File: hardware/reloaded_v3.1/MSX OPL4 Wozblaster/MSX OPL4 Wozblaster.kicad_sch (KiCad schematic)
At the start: 34 parts, among them IC1 GAL16V8D, IC2 KM684000ALG, IC3 KM684000ALG, IC4 NJM4558, IC5 YMF278B-F, IC6 AM29F016B-120EC, Q1 33.8688, SW1 SW_Push, U1 KCX_BT_EMITTER, U2 UDA1334MOD

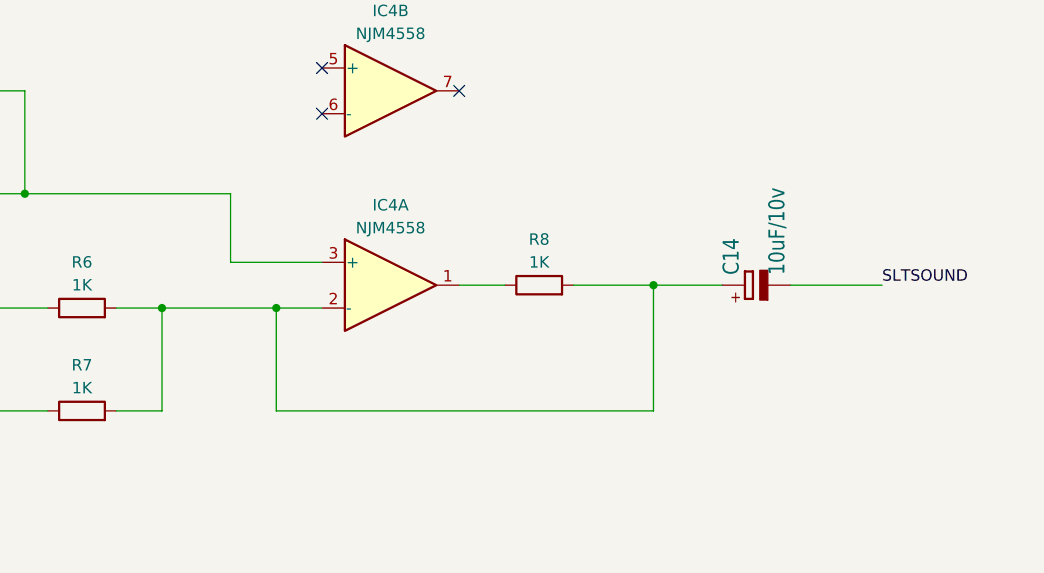
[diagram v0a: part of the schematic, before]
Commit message: v3.2
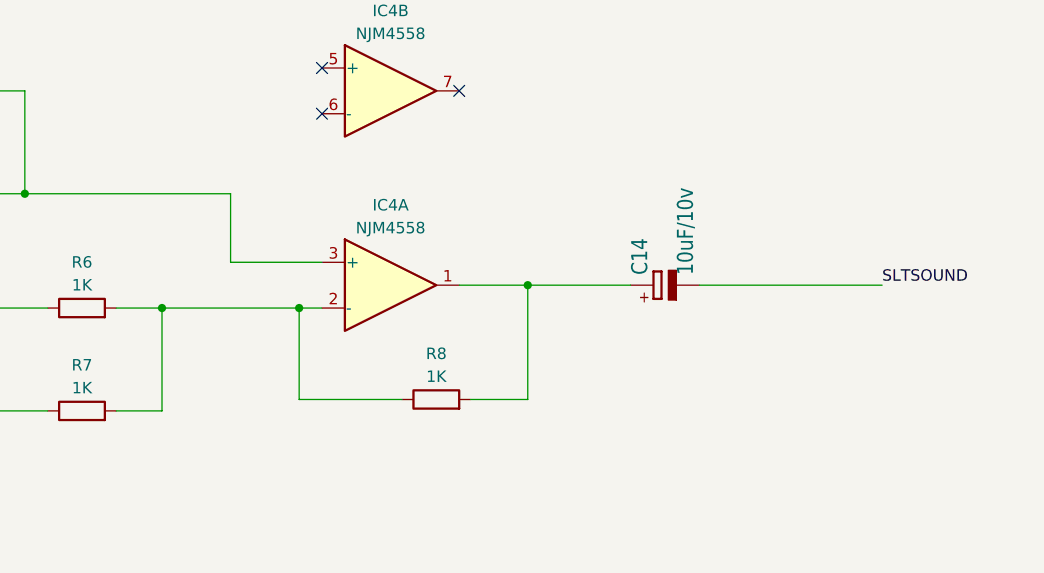
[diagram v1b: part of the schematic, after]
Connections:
- net at IC4.1: now also C14.1 (+), R8.2; no longer R8.1
- net at IC4.2 (-), R6.2, R7.2: now also R8.1; no longer C14.1 (+), R8.2
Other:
- moved on the sheet: C14
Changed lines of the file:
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@@
     (comment 4 "Wozblaster Reloaded v3")
   )
+  (junction (at 452.12 252.73) (diameter 0) (color 0 0 0 0)
+  )
   (junction (at 157.48 288.29) (diameter 0) (color 0 0 0 0)
   )
@@
   (junction (at 234.95 139.7) (diameter 0) (color 0 0 0 0)
   )
-  (junction (at 449.58 252.73) (diameter 0) (color 0 0 0 0)
-  )
   (junction (at 200.66 149.86) (diameter 0) (color 0 0 0 0)
   )
+  (junction (at 477.52 250.19) (diameter 0) (color 0 0 0 0)
+  )
   (junction (at 224.79 118.11) (diameter 0) (color 0 0 0 0)
   )
@@
   (junction (at 234.95 152.4) (diameter 0) (color 0 0 0 0)
   )
-  (junction (at 491.49 250.19) (diameter 0) (color 0 0 0 0)
-  )
   (junction (at 214.63 118.11) (diameter 0) (color 0 0 0 0)
   )
@@
     (stroke (width 0) (type default))
   )
-  (wire (pts (xy 436.88 252.73) (xy 449.58 252.73))
+  (wire (pts (xy 436.88 252.73) (xy 452.12 252.73))
     (stroke (width 0) (type default))
   )
@@
     (stroke (width 0) (type default))
   )
+  (wire (pts (xy 471.17 262.89) (xy 477.52 262.89))
+    (stroke (width 0) (type default))
+  )
   (wire (pts (xy 421.64 228.6) (xy 421.64 240.03))
     (stroke (width 0) (type default))
@@
     (stroke (width 0) (type default))
   )
-  (wire (pts (xy 491.49 250.19) (xy 499.11 250.19))
-    (stroke (width 0) (type default))
-  )
   (wire (pts (xy 396.24 228.6) (xy 405.13 228.6))
     (stroke (width 0) (type default))
@@
     (stroke (width 0) (type default))
   )
+  (wire (pts (xy 452.12 262.89) (xy 463.55 262.89))
+    (stroke (width 0) (type default))
+  )
   (wire (pts (xy 496.57 76.2) (xy 502.92 76.2))
     (stroke (width 0) (type default))
@@
     (stroke (width 0) (type default))
   )
+  (wire (pts (xy 477.52 250.19) (xy 488.95 250.19))
+    (stroke (width 0) (type default))
+  )
   (wire (pts (xy 273.05 147.32) (xy 278.13 147.32))
     (stroke (width 0) (type default))
@@
     (stroke (width 0) (type default))
   )
-  (wire (pts (xy 469.9 250.19) (xy 474.98 250.19))
+  (wire (pts (xy 469.9 250.19) (xy 477.52 250.19))
     (stroke (width 0) (type default))
   )
@@
     (stroke (width 0) (type default))
   )
-  (wire (pts (xy 482.6 250.19) (xy 491.49 250.19))
-    (stroke (width 0) (type default))
-  )
   (wire (pts (xy 273.05 109.22) (xy 278.13 109.22))
     (stroke (width 0) (type default))
@@
     (stroke (width 0) (type default))
   )
+  (wire (pts (xy 477.52 262.89) (xy 477.52 250.19))
+    (stroke (width 0) (type default))
+  )
   (wire (pts (xy 132.08 270.51) (xy 127 270.51))
     (stroke (width 0) (type default))
@@
     (stroke (width 0) (type default))
   )
-  (wire (pts (xy 506.73 250.19) (xy 516.89 250.19))
-    (stroke (width 0) (type default))
-  )
   (wire (pts (xy 381 273.05) (xy 387.35 273.05))
     (stroke (width 0) (type default))
@@
     (stroke (width 0) (type default))
   )
-  (wire (pts (xy 491.49 250.19) (xy 491.49 264.16))
-    (stroke (width 0) (type default))
-  )
   (wire (pts (xy 217.17 54.61) (xy 229.87 54.61))
     (stroke (width 0) (type default))
@@
     (stroke (width 0) (type default))
   )
+  (wire (pts (xy 452.12 252.73) (xy 454.66 252.73))
+    (stroke (width 0) (type default))
+  )
   (wire (pts (xy 314.96 118.11) (xy 321.31 118.11))
     (stroke (width 0) (type default))
@@
     (stroke (width 0) (type default))
   )
-  (wire (pts (xy 449.58 264.16) (xy 449.58 252.73))
+  (wire (pts (xy 452.12 252.73) (xy 452.12 262.89))
     (stroke (width 0) (type default))
   )
@@
     (stroke (width 0) (type default))
   )
-  (wire (pts (xy 449.58 252.73) (xy 454.66 252.73))
-    (stroke (width 0) (type default))
-  )
   (wire (pts (xy 381 270.51) (xy 383.54 270.51))
     (stroke (width 0) (type default))
@@
     (stroke (width 0) (type default))
   )
-  (wire (pts (xy 491.49 264.16) (xy 449.58 264.16))
-    (stroke (width 0) (type default))
-  )
   (wire (pts (xy 273.05 269.24) (xy 285.75 269.24))
     (stroke (width 0) (type default))
@@
     (stroke (width 0) (type default))
   )
+  (wire (pts (xy 496.57 250.19) (xy 516.89 250.19))
+    (stroke (width 0) (type default))
+  )
   (wire (pts (xy 496.57 81.28) (xy 502.92 81.28))
     (stroke (width 0) (type default))
@@
     )
   )
-  (symbol (lib_id "Device:R") (at 478.79 250.19 90) (unit 1)
-    (in_bom yes) (on_board yes) (dnp no) (fields_autoplaced)
-    (property "Reference" "R8" (at 478.79 245.11 90)
-      (effects (font (size 1.27 1.27)))
-    )
-    (property "Value" "1K" (at 478.79 247.65 90)
-      (effects (font (size 1.27 1.27)))
-    )
-    (property "Footprint" "Resistor_SMD:R_0603_1608Metric" (at 478.79 251.968 90)
-      (effects (font (size 1.27 1.27)) hide)
-    )
-    (property "Datasheet" "~" (at 478.79 250.19 0)
-      (effects (font (size 1.27 1.27)) hide)
-    )
-    (pin "1")
-    (pin "2")
-    (instances
-      (project "MSX OPL4 Wozblaster"
-        (path "/319085e4-dbf0-404d-8e32-9614d4e1a0c6"
-          (reference "R8") (unit 1)
-        )
-      )
-    )
-  )
   (symbol (lib_id "power:GND") (at 90.17 293.37 0) (unit 1)
     (in_bom yes) (on_board yes) (dnp no) (fields_autoplaced)
@@
     )
   )
+  (symbol (lib_id "Device:R") (at 467.36 262.89 90) (unit 1)
+    (in_bom yes) (on_board yes) (dnp no) (fields_autoplaced)
+    (property "Reference" "R8" (at 467.36 257.81 90)
+      (effects (font (size 1.27 1.27)))
+    )
+    (property "Value" "1K" (at 467.36 260.35 90)
+      (effects (font (size 1.27 1.27)))
+    )
+    (property "Footprint" "Resistor_SMD:R_0603_1608Metric" (at 467.36 264.668 90)
+      (effects (font (size 1.27 1.27)) hide)
+    )
+    (property "Datasheet" "~" (at 467.36 262.89 0)
+      (effects (font (size 1.27 1.27)) hide)
+    )
+    (pin "1")
+    (pin "2")
+    (instances
+      (project "MSX OPL4 Wozblaster"
+        (path "/319085e4-dbf0-404d-8e32-9614d4e1a0c6"
+          (reference "R8") (unit 1)
+        )
+      )
+    )
+  )
   (symbol (lib_id "CRISAG:C-EU") (at 208.28 118.11 270) (unit 1)
     (in_bom yes) (on_board yes) (dnp no)
@@
     )
   )
-  (symbol (lib_id "CRISAG:CPOLSMCB") (at 501.65 250.19 90) (unit 1)
+  (symbol (lib_id "CRISAG:CPOLSMCB") (at 491.49 250.19 90) (unit 1)
     (in_bom yes) (on_board yes) (dnp no)
-    (property "Reference" "C14" (at 501.1674 249.047 0)
+    (property "Reference" "C14" (at 491.0074 249.047 0)
       (effects (font (size 1.778 1.5113)) (justify left bottom))
     )
-    (property "Value" "10uF/10v" (at 506.2474 249.047 0)
+    (property "Value" "10uF/10v" (at 496.0874 249.047 0)
       (effects (font (size 1.778 1.5113)) (justify left bottom))
     )
-    (property "Footprint" "Capacitor_Tantalum_SMD:CP_EIA-3216-18_Kemet-A" (at 501.65 250.19 0)
+    (property "Footprint" "Capacitor_Tantalum_SMD:CP_EIA-3216-18_Kemet-A" (at 491.49 250.19 0)
       (effects (font (size 1.27 1.27)) hide)
     )
-    (property "Datasheet" "" (at 501.65 250.19 0)
+    (property "Datasheet" "" (at 491.49 250.19 0)
       (effects (font (size 1.27 1.27)) hide)
     )
